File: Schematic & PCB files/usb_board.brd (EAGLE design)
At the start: 145 x 38.4 mm, 2 parts, among them J1 USB4115-03-C_REVA, X1 BM04B-SRSS-TB

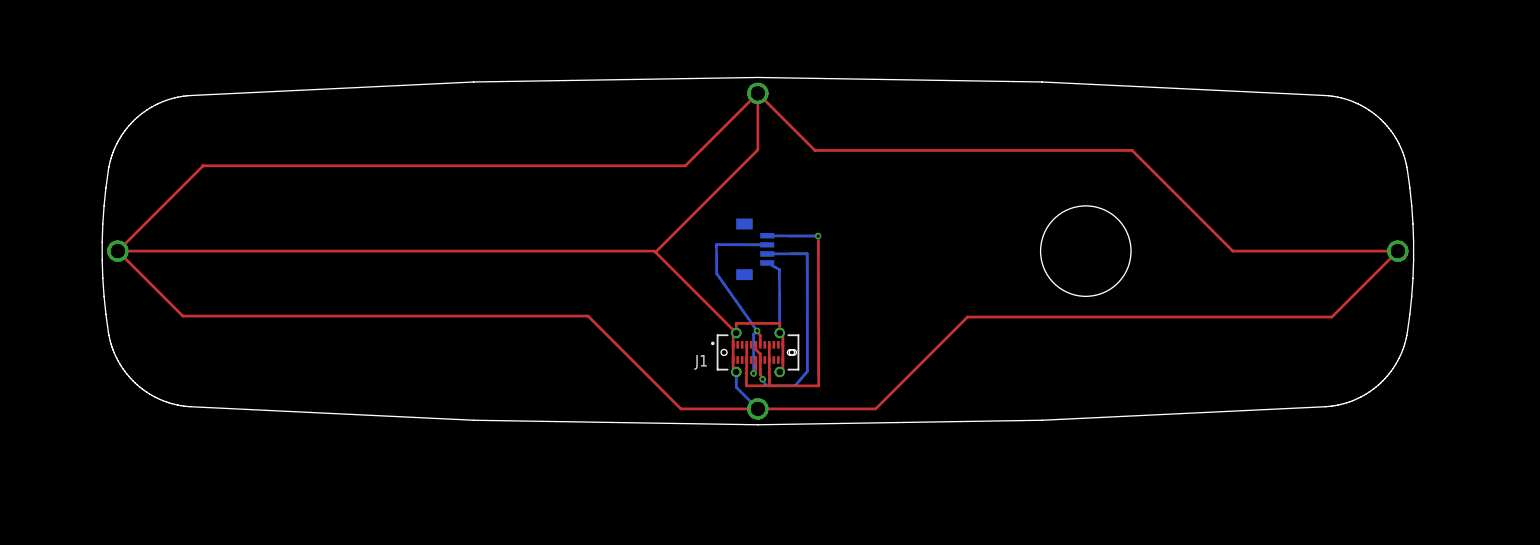
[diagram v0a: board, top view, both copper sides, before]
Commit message: Updated EAGLE files
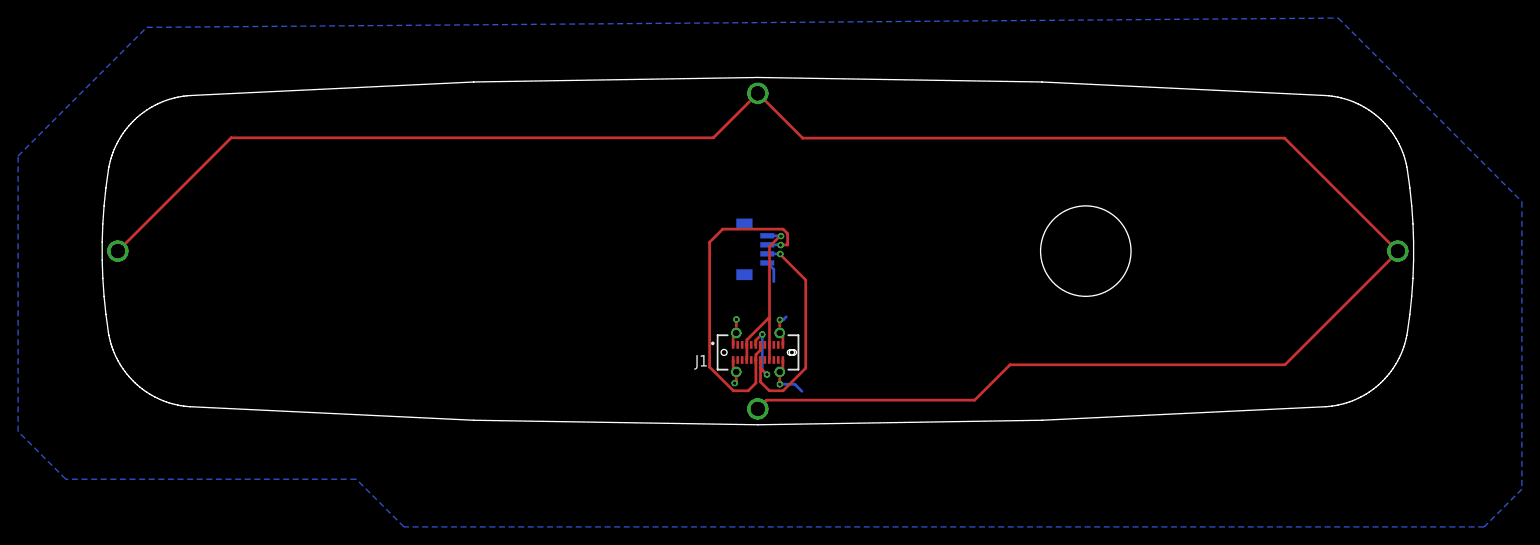
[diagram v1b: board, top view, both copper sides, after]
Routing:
- net GND: track 436.1 -> 17.5 mm
- net AGND: track 0.00 -> 234.0 mm, vias 0 -> 4
- net VCC: track 39.3 -> 21.6 mm
- net D-: track 24.7 -> 37.8 mm, vias 2 -> 1
- net D+: track 27.6 -> 31.2 mm, vias 1 -> 3
- added copper zone on layer 16, net GND
